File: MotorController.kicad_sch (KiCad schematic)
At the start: 129 parts, among them IC1 ft234xd, IC2 A3921KLPTR-T, IC3 A3921KLPTR-T, J1 SH, J10 XT, J11 XT30, J2 USB_B_Micro, J3 Conn_01x02, J4 Conn_01x04, J5 3020-10-0300-00, J6 SH, J7 SH, J8 3020-10-0300-00, J9 Conn_01x02, Q1 GSFQ6806, Q2 GSFQ6806, Q3 GSFQ6806, Q4 SFS9Z34, Q5 GSFQ6806, Q6 SFS9Z34, SW2 SW_MEC_5E, SW3 SW_MEC_5E, SW4 SW_SPDT, SW5 SW_MEC_5E, U1 LXES11D, U2 STM32F303K8Tx, U3 TJA1441AT, U4 TPSM13604HNDWR, U5 LMZ12002EXT, Y1 32M

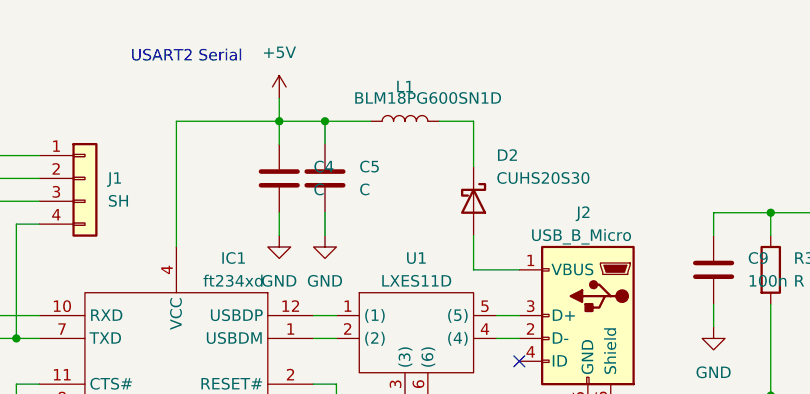
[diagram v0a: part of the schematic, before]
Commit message: フットプリント再更新
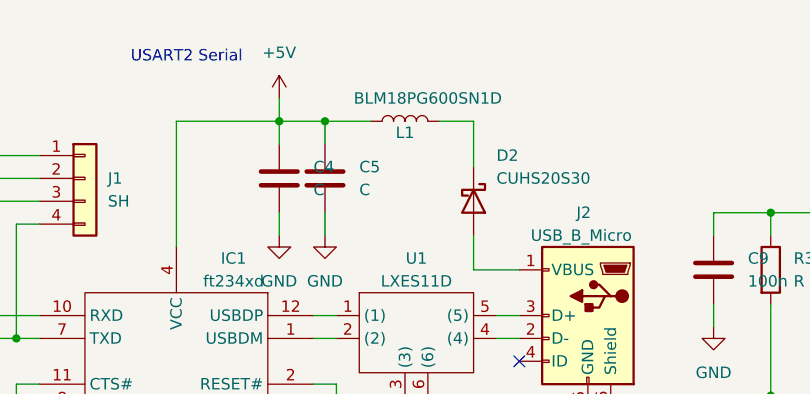
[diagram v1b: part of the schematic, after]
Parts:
- Q1, Q2, Q3, Q5: footprint (none) -> Package_SO:HSOP-8-1EP_3.9x4.9mm_P1.27mm_EP2.3x2.3mm
- R1, R10, R11, R12, R13, R14, R15, R16, R17, R18, R19, R2, R20, R21, R22, R23, R24, R25, R26, R27, R28, R29, R3, R30, R31, R32, R33, R34, R35, R36, R37, R38, R39, R4, R40, R41, R42, R43, R5, R6, R7, R8, R9: footprint (none) -> Resistor_SMD:R_0603_1608Metric
- U1: footprint (none) -> LibraryLoader:LXES11DAA2135
- U4, U5: footprint (none) -> Package_TO_SOT_SMD:Texas_NDW-7_TabPin8
